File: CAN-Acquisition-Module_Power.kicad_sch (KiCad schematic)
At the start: 23 parts

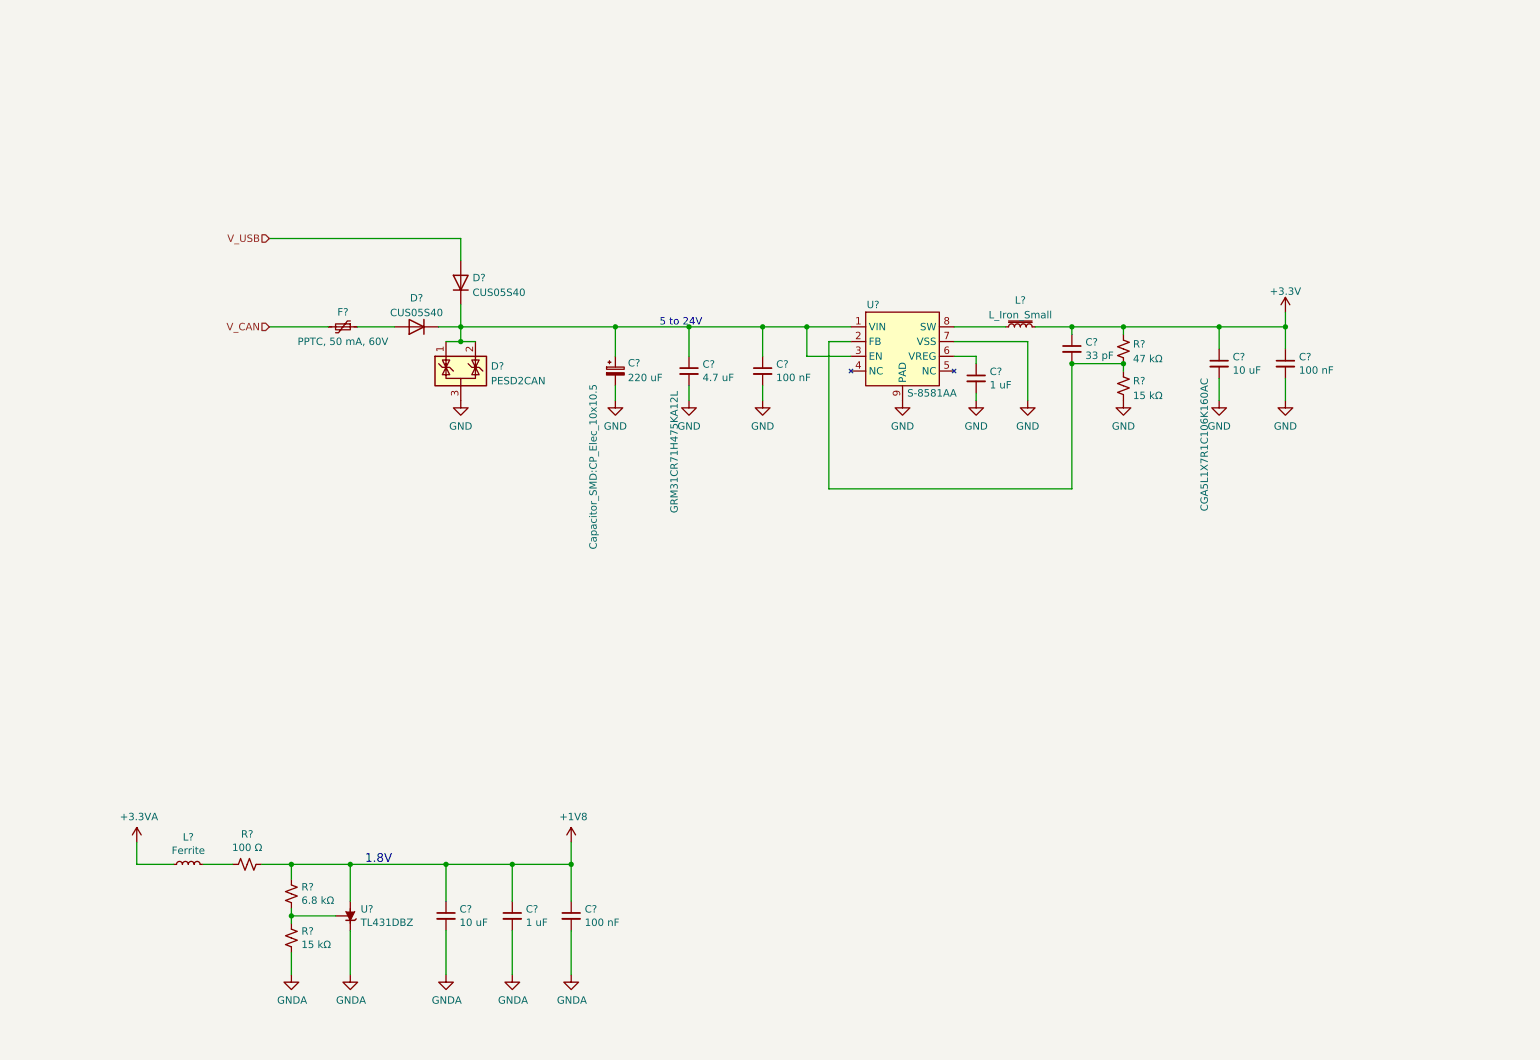
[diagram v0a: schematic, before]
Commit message: Added stuff and cleanup
Added LED, Power outputs, additional descriptions
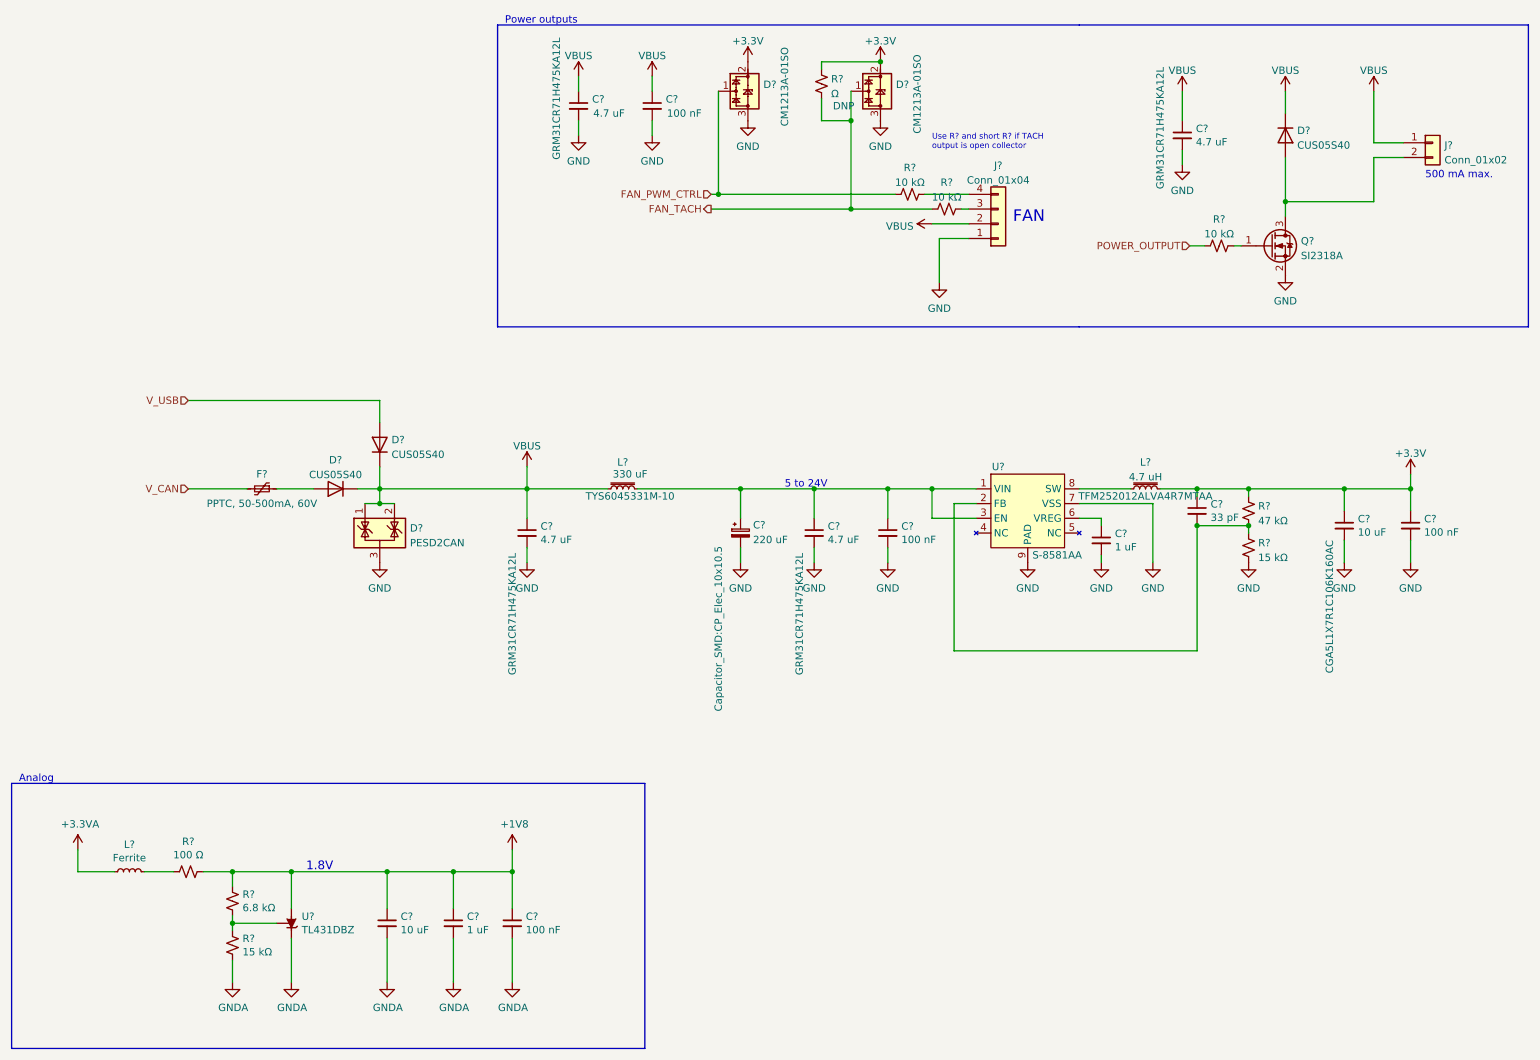
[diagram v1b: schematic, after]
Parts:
- added C? (x3): 4.7 uF, Capacitor_SMD:C_1206_3216Metric, symbol Device:C_Small
- added C?: 100 nF, Capacitor_SMD:C_0603_1608Metric, symbol Device:C_Small
- added D?: CUS05S40, CAN-Acquisition-Module:Toshiba_USC, symbol Device:D
- added D? (x2): CM1213A-01SO, Package_TO_SOT_SMD:SOT-23, symbol Power_Protection:CM1213A-01SO
- added J?: Conn_01x02, Connector_PinHeader_2.54mm:PinHeader_1x02_P2.54mm_Vertical, symbol Connector_Generic:Conn_01x02
- added J?: Conn_01x04, Connector:FanPinHeader_1x04_P2.54mm_Vertical, symbol Connector_Generic:Conn_01x04
- added L?: 330 uF, Inductor_SMD:L_Bourns_SRN6045TA, symbol Device:L_Iron_Small
- added Q?: SI2318A, Package_TO_SOT_SMD:SOT-23, symbol Transistor_FET:2N7002K
- added R?: Ω, Resistor_SMD:R_0603_1608Metric, symbol Device:R_Small_US
- added R? (x3): 10 kΩ, Resistor_SMD:R_0603_1608Metric, symbol Device:R_Small_US
- F?: value PPTC, 50 mA, 60V -> PPTC, 50-500mA, 60V
- L?: value L_Iron_Small -> 4.7 uH; MPN (none) -> TFM252012ALVA4R7MTAA
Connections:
- net +3V3: now also D?.2 (VP), D?.2 (VP), R?.2
- net GND: now also C?.2, C?.2, C?.2, C?.2, D?.3 (VN), D?.3 (VN), J?.1 (Pin_1), Q?.2 (S)
- net at C?.1, C?.1, C?.1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: now also L?.2; no longer D?.1 (K), D?.1 (K), D?.1 (K), D?.2 (K)
- new net: D?.2 (A), J?.2 (Pin_2), Q?.3 (D)
- new net: J?.4 (Pin_4), R?.2
- new net: J?.3 (Pin_3), R?.2
- new net: Q?.1 (G), R?.2
- new net FAN_PWM_CTRL: D?.1 (CH1), R?.1
- new net FAN_TACH: D?.1 (CH1), R?.1, R?.1
- new net POWER_OUTPUT: R?.1
- new net VBUS: C?.1, C?.1, C?.1, C?.1, D?.1 (K), D?.1 (K), D?.1 (K), D?.1 (K), D?.2 (K), J?.1 (Pin_1), J?.2 (Pin_2), L?.1
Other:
- note added: "500 mA max."
- note added: "Analog"
- note added: "FAN"
- note added: "Power outputs"
- note added: "Use R? and short R? if TACH output is open collector"
- moved on the sheet: C?, D?, F?, L?, R?, U?
